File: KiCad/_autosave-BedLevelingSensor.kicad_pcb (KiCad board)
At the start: 2 copper layers, 11.2 x 19.7 mm, 9 parts, among them J1 SOLENOID, J2 Sensor, J3 Input, U1 ATTINY15-1SC, U2 L9110

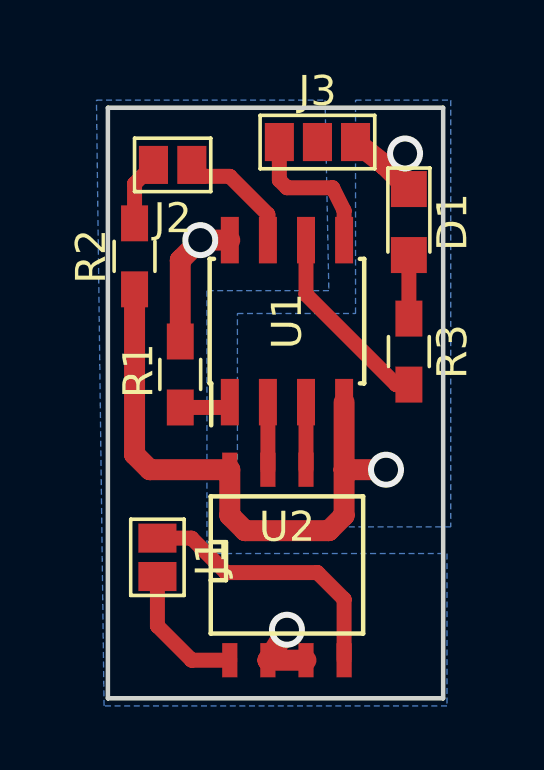
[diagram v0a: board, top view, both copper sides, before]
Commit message: Schematic and PCB
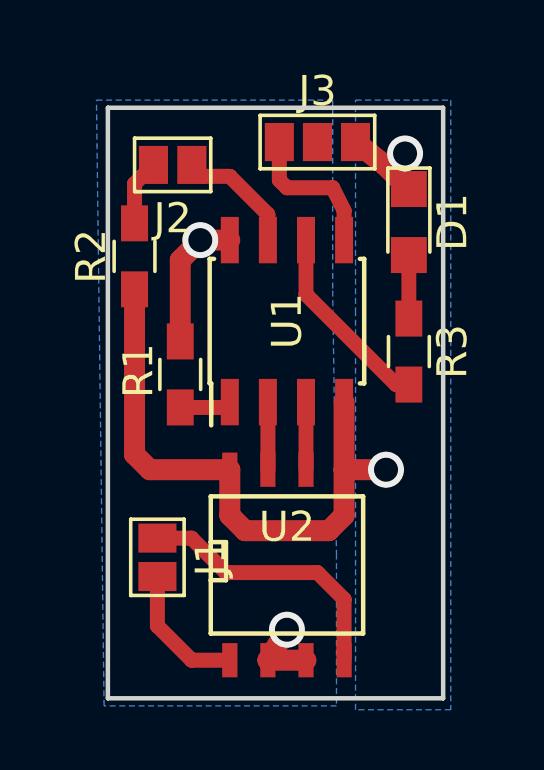
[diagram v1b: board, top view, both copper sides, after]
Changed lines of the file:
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@@
     (links 19)
     (no_connects 1)
-    (area 132.004999 106.731999 143.331001 125.932001)
+    (area 130.544 104.64 144.638 126.111001)
     (thickness 1.6)
     (drawings 4)
@@
     (visible_elements 7FFFFFFF)
     (pcbplotparams
-      (layerselection 0x00030_80000001)
+      (layerselection 0x01000_00000001)
       (usegerberextensions false)
-      (excludeedgelayer true)
+      (excludeedgelayer false)
       (linewidth 0.100000)
       (plotframeref false)
@@
       (padsonsilk false)
       (subtractmaskfromsilk false)
-      (outputformat 1)
+      (outputformat 3)
       (mirror false)
-      (drillshape 1)
+      (drillshape 2)
       (scaleselection 1)
       (outputdirectory ""))
@@
     (polygon
       (pts
-        (xy 143.383 126.111) (xy 131.953 126.111) (xy 131.699 105.918) (xy 139.319 105.918) (xy 139.446 112.268)
-        (xy 135.382 112.268) (xy 135.382 121.031) (xy 143.383 121.031)
+        (xy 139.573 112.268) (xy 139.7 121.031) (xy 139.7 126.111) (xy 131.953 126.111) (xy 131.699 105.918)
+        (xy 139.573 105.918)
       )
     )
@@
     (polygon
       (pts
-        (xy 143.51 120.142) (xy 136.398 120.142) (xy 136.398 113.03) (xy 140.335 113.03) (xy 140.335 105.918)
+        (xy 143.51 126.238) (xy 140.335 126.238) (xy 140.335 113.03) (xy 140.335 113.03) (xy 140.335 105.918)
         (xy 143.51 105.918)
       )
